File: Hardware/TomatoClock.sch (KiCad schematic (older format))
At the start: 26 parts, among them J1 Boot, J2 UART, J3 USB_B_Micro, J4 Ultrasonic, J5 Buttons, J6 Battery, Q1 S9014, U1 STM32F103C8T6, U2 WS4518E, U3 AP1117-33, Y1 8MHz, Y2 32.768kHz

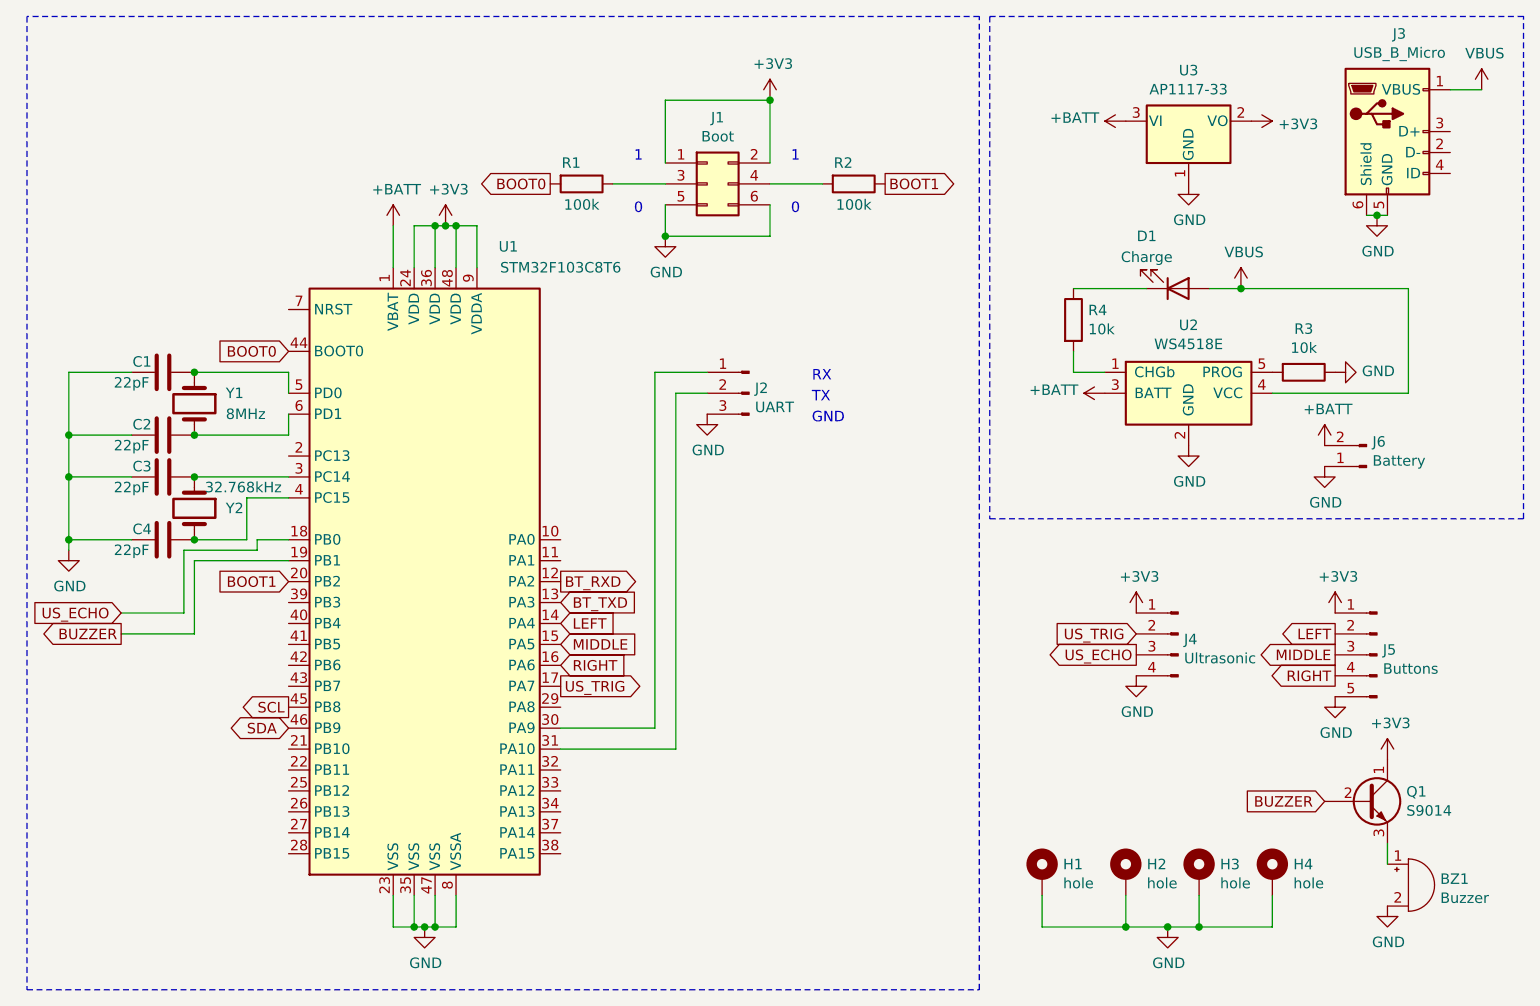
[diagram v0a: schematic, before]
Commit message: Hardware: Update PCB and schematics
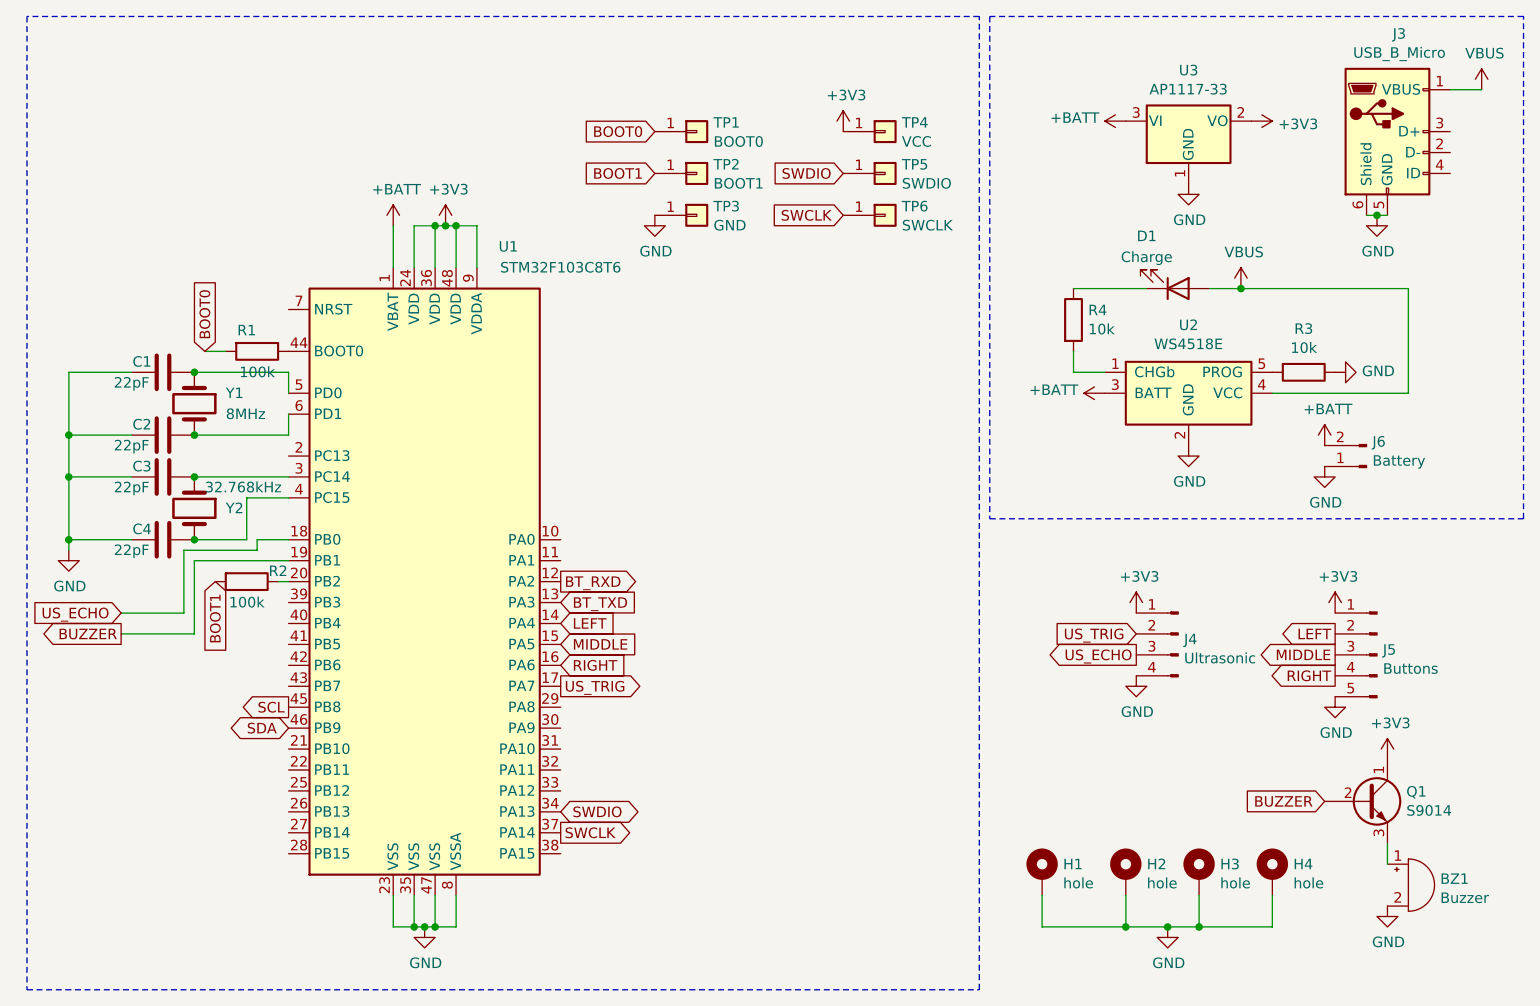
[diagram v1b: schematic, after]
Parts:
- removed J1: Boot, Connector_PinHeader_2.00mm:PinHeader_2x03_P2.00mm_Vertical, symbol Connector_Generic:Conn_02x03_Odd_Even
- removed J2: UART, Connector_PinHeader_2.00mm:PinHeader_1x03_P2.00mm_Vertical, symbol Connector:Conn_01x03_Male
- added TP1: BOOT0, TestPoint:TestPoint_Pad_D1.5mm, symbol Connector_Generic:Conn_01x01
- added TP2: BOOT1, TestPoint:TestPoint_Pad_D1.5mm, symbol Connector_Generic:Conn_01x01
- added TP3: GND, TestPoint:TestPoint_Pad_D1.5mm, symbol Connector_Generic:Conn_01x01
- added TP4: VCC, TestPoint:TestPoint_Pad_D1.5mm, symbol Connector_Generic:Conn_01x01
- added TP5: SWDIO, TestPoint:TestPoint_Pad_D1.5mm, symbol Connector_Generic:Conn_01x01
- added TP6: SWCLK, TestPoint:TestPoint_Pad_D1.5mm, symbol Connector_Generic:Conn_01x01
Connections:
- net +3V3: now also TP4.1 (Pin_1)
- net BOOT0: now also TP1.1 (Pin_1); no longer U1.44 (BOOT0)
- net BOOT1: now also R2.2, TP2.1 (Pin_1); no longer R2.1, U1.20 (PB2)
- net GND: now also TP3.1 (Pin_1)
- net SWDIO: now reaches U1.34 (PA13)
- net SWDIO: now also TP5.1 (Pin_1)
- net SWCLK: now reaches U1.37 (PA14)
- net SWCLK: now also TP6.1 (Pin_1)
- net at R1.1: now also U1.44 (BOOT0)
- new net: R2.1, U1.20 (PB2)
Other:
- note removed: "0"
- note removed: "1"
- note removed: "GND"
- note removed: "RX"
- note removed: "TX"
- moved on the sheet: R1
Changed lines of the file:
@@
 	1600 3050 1350 3050
 Connection ~ 1350 3050
-Text GLabel 1800 2150 0    50   Input ~ 0
+Text GLabel 1400 2150 1    50   Input ~ 0
 BOOT0
-Text GLabel 1800 3250 0    50   Input ~ 0
+Text GLabel 1450 3250 3    50   Input ~ 0
 BOOT1
-$Comp
-L Device:R R2
-U 1 1 61A5B290
-P 4500 1350
-F 0 "R2" V 4400 1300 50  0000 C CNN
-F 1 "100k" V 4600 1350 50  0000 C CNN
-F 2 "Resistor_SMD:R_0603_1608Metric" V 4430 1350 50  0001 C CNN
-F 3 "~" H 4500 1350 50  0001 C CNN
-	1    4500 1350
-	0    1    1    0
-$EndComp
-Wire Wire Line
-	3350 1350 3600 1350
-Wire Wire Line
-	4100 1350 4350 1350
-Text GLabel 3050 1350 0    50   Output ~ 0
-BOOT0
-Text GLabel 4650 1350 2    50   Output ~ 0
-BOOT1
-$Comp
-L power:+3V3 #PWR06
-U 1 1 61A612C6
-P 4100 950
-F 0 "#PWR06" H 4100 800 50  0001 C CNN
-F 1 "+3V3" H 4115 1123 50  0000 C CNN
-F 2 "" H 4100 950 50  0001 C CNN
-F 3 "" H 4100 950 50  0001 C CNN
-	1    4100 950
-	1    0    0    -1
-$EndComp
-Wire Wire Line
-	4100 950  4100 1250
-Wire Wire Line
-	4100 950  3600 950
-Wire Wire Line
-	3600 950  3600 1250
-Connection ~ 4100 950
-$Comp
-L power:GND #PWR05
-U 1 1 61A66348
-P 3600 1600
-F 0 "#PWR05" H 3600 1350 50  0001 C CNN
-F 1 "GND" H 3605 1427 50  0000 C CNN
-F 2 "" H 3600 1600 50  0001 C CNN
-F 3 "" H 3600 1600 50  0001 C CNN
-	1    3600 1600
-	1    0    0    -1
-$EndComp
-Wire Wire Line
-	3600 1450 3600 1600
-Wire Wire Line
-	4100 1450 4100 1600
-Wire Wire Line
-	4100 1600 3600 1600
-Connection ~ 3600 1600
 $Comp
 L Regulator_Linear:AP1117-33 U3
@@
 	1    0    0    -1
 $EndComp
-$Comp
-L Connector:Conn_01x03_Male J2
-U 1 1 61A91DE9
-P 4000 2350
-F 0 "J2" H 3972 2374 50  0000 R CNN
-F 1 "UART" H 3972 2283 50  0000 R CNN
-F 2 "Connector_PinHeader_2.00mm:PinHeader_1x03_P2.00mm_Vertical" H 4000 2350 50  0001 C CNN
-F 3 "~" H 4000 2350 50  0001 C CNN
-	1    4000 2350
-	-1   0    0    -1
-$EndComp
-$Comp
-L power:GND #PWR014
-U 1 1 61A954C1
-P 3800 2450
-F 0 "#PWR014" H 3800 2200 50  0001 C CNN
-F 1 "GND" H 3805 2277 50  0000 C CNN
-F 2 "" H 3800 2450 50  0001 C CNN
-F 3 "" H 3800 2450 50  0001 C CNN
-	1    3800 2450
-	1    0    0    -1
-$EndComp
-Text Notes 3450 1500 0    50   ~ 0
-0
-Text Notes 3450 1250 0    50   ~ 0
-1
-Text Notes 4200 1500 0    50   ~ 0
-0
-Text Notes 4200 1250 0    50   ~ 0
-1
-Wire Wire Line
-	3100 3950 3550 3950
-Wire Wire Line
-	3550 3950 3550 2250
-Wire Wire Line
-	3550 2250 3800 2250
-Wire Wire Line
-	3800 2350 3650 2350
-Wire Wire Line
-	3650 2350 3650 4050
-Wire Wire Line
-	3650 4050 3100 4050
-Text Notes 4300 2300 0    50   ~ 0
-RX
-Text Notes 4300 2400 0    50   ~ 0
-TX
-Text Notes 4300 2500 0    50   ~ 0
-GND
 Wire Notes Line
 	550  550  550  5200
@@
 L Device:R R1
 U 1 1 61A5A591
-P 3200 1350
-F 0 "R1" V 3100 1300 50  0000 C CNN
-F 1 "100k" V 3300 1350 50  0000 C CNN
-F 2 "Resistor_SMD:R_0603_1608Metric" V 3130 1350 50  0001 C CNN
-F 3 "~" H 3200 1350 50  0001 C CNN
-	1    3200 1350
+P 1650 2150
+F 0 "R1" V 1550 2100 50  0000 C CNN
+F 1 "100k" V 1750 2150 50  0000 C CNN
+F 2 "Resistor_SMD:R_0603_1608Metric" V 1580 2150 50  0001 C CNN
+F 3 "~" H 1650 2150 50  0001 C CNN
+	1    1650 2150
 	0    1    1    0
-$EndComp
-$Comp
-L Connector_Generic:Conn_02x03_Odd_Even J1
-U 1 1 61ACA0B6
-P 3800 1350
-F 0 "J1" H 3850 1667 50  0000 C CNN
-F 1 "Boot" H 3850 1576 50  0000 C CNN
-F 2 "Connector_PinHeader_2.00mm:PinHeader_2x03_P2.00mm_Vertical" H 3800 1350 50  0001 C CNN
-F 3 "~" H 3800 1350 50  0001 C CNN
-	1    3800 1350
-	1    0    0    -1
 $EndComp
 $Comp
@@
 	1    0    0    -1
 $EndComp
+Wire Wire Line
+	1500 2150 1400 2150
+$Comp
+L Device:R R2
+U 1 1 61C1663A
+P 1600 3250
+F 0 "R2" V 1550 3400 50  0000 C CNN
+F 1 "100k" V 1700 3250 50  0000 C CNN
+F 2 "Resistor_SMD:R_0603_1608Metric" V 1530 3250 50  0001 C CNN
+F 3 "~" H 1600 3250 50  0001 C CNN
+	1    1600 3250
+	0    1    1    0
+$EndComp
+Wire Wire Line
+	1800 3250 1750 3250
+$Comp
+L Connector_Generic:Conn_01x01 TP1
+U 1 1 61BF10E0
+P 3750 1100
+F 0 "TP1" H 3830 1142 50  0000 L CNN
+F 1 "BOOT0" H 3830 1051 50  0000 L CNN
+F 2 "TestPoint:TestPoint_Pad_D1.5mm" H 3750 1100 50  0001 C CNN
+F 3 "~" H 3750 1100 50  0001 C CNN
+	1    3750 1100
+	1    0    0    -1
+$EndComp
+Text GLabel 3550 1100 0    50   Input ~ 0
+BOOT0
+$Comp
+L Connector_Generic:Conn_01x01 TP2
+U 1 1 61BF32BB
+P 3750 1300
+F 0 "TP2" H 3830 1342 50  0000 L CNN
+F 1 "BOOT1" H 3830 1251 50  0000 L CNN
+F 2 "TestPoint:TestPoint_Pad_D1.5mm" H 3750 1300 50  0001 C CNN
+F 3 "~" H 3750 1300 50  0001 C CNN
+	1    3750 1300
+	1    0    0    -1
+$EndComp
+Text GLabel 3550 1300 0    50   Input ~ 0
+BOOT1
+$Comp
+L Connector_Generic:Conn_01x01 TP3
+U 1 1 61BF5138
+P 3750 1500
+F 0 "TP3" H 3830 1542 50  0000 L CNN
+F 1 "GND" H 3830 1451 50  0000 L CNN
+F 2 "TestPoint:TestPoint_Pad_D1.5mm" H 3750 1500 50  0001 C CNN
+F 3 "~" H 3750 1500 50  0001 C CNN
+	1    3750 1500
+	1    0    0    -1
+$EndComp
+$Comp
+L power:GND #PWR05
+U 1 1 61BF6FB1
+P 3550 1500
+F 0 "#PWR05" H 3550 1250 50  0001 C CNN
+F 1 "GND" H 3555 1327 50  0000 C CNN
+F 2 "" H 3550 1500 50  0001 C CNN
+F 3 "" H 3550 1500 50  0001 C CNN
+	1    3550 1500
+	1    0    0    -1
+$EndComp
+$Comp
+L Connector_Generic:Conn_01x01 TP4
+U 1 1 61BF77FB
+P 4650 1100
+F 0 "TP4" H 4730 1142 50  0000 L CNN
+F 1 "VCC" H 4730 1051 50  0000 L CNN
+F 2 "TestPoint:TestPoint_Pad_D1.5mm" H 4650 1100 50  0001 C CNN
+F 3 "~" H 4650 1100 50  0001 C CNN
+	1    4650 1100
+	1    0    0    -1
+$EndComp
+$Comp
+L power:+3V3 #PWR06
+U 1 1 61BF9632
+P 4450 1100
+F 0 "#PWR06" H 4450 950 50  0001 C CNN
+F 1 "+3V3" H 4465 1273 50  0000 C CNN
+F 2 "" H 4450 1100 50  0001 C CNN
+F 3 "" H 4450 1100 50  0001 C CNN
+	1    4450 1100
+	1    0    0    -1
+$EndComp
+Text GLabel 3100 4350 2    50   BiDi ~ 0
+SWDIO
+Text GLabel 3100 4450 2    50   Output ~ 0
+SWCLK
+$Comp
+L Connector_Generic:Conn_01x01 TP5
+U 1 1 61BF3A3F
+P 4650 1300
+F 0 "TP5" H 4730 1342 50  0000 L CNN
+F 1 "SWDIO" H 4730 1251 50  0000 L CNN
+F 2 "TestPoint:TestPoint_Pad_D1.5mm" H 4650 1300 50  0001 C CNN
+F 3 "~" H 4650 1300 50  0001 C CNN
+	1    4650 1300
+	1    0    0    -1
+$EndComp
+Text GLabel 4450 1300 0    50   Input ~ 0
+SWDIO
+$Comp
+L Connector_Generic:Conn_01x01 TP6
+U 1 1 61BF57EE
+P 4650 1500
+F 0 "TP6" H 4730 1542 50  0000 L CNN
+F 1 "SWCLK" H 4730 1451 50  0000 L CNN
+F 2 "TestPoint:TestPoint_Pad_D1.5mm" H 4650 1500 50  0001 C CNN
+F 3 "~" H 4650 1500 50  0001 C CNN
+	1    4650 1500
+	1    0    0    -1
+$EndComp
+Text GLabel 4450 1500 0    50   Input ~ 0
+SWCLK
 $EndSCHEMATC

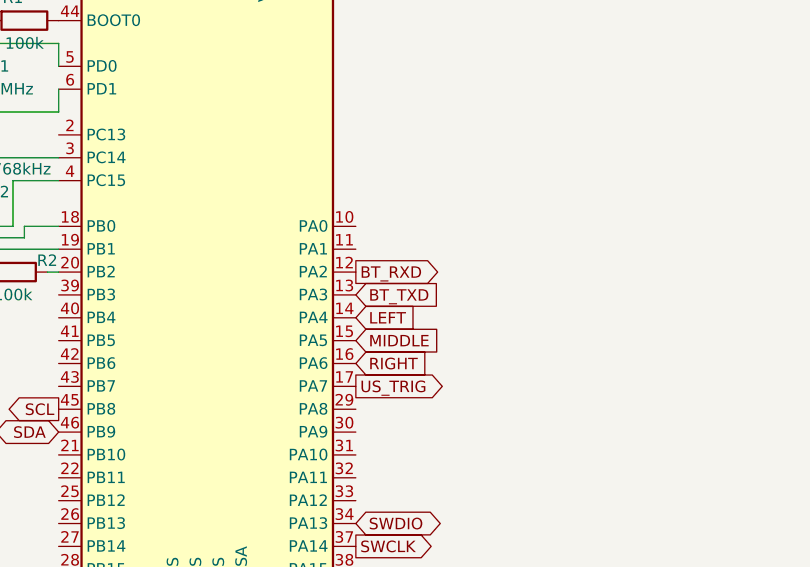
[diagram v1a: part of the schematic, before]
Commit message: Hardware: Update hardware
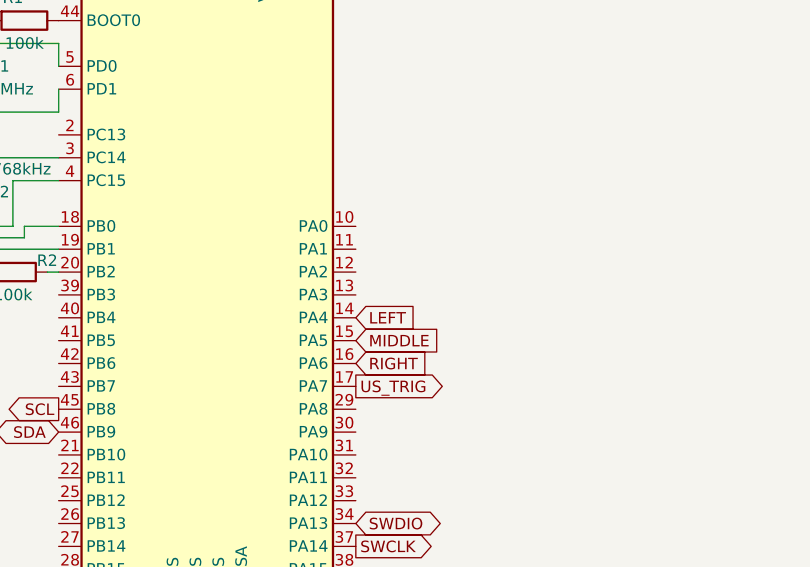
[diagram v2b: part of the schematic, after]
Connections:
- net BT_RXD: no longer names the net of U1.12 (PA2)
- net BT_TXD: no longer names the net of U1.13 (PA3)
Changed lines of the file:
@@
 Text GLabel 6800 3700 0    50   Output ~ 0
 RIGHT
-Text GLabel 3100 3250 2    50   Output ~ 0
-BT_RXD
-Text GLabel 3100 3350 2    50   Input ~ 0
-BT_TXD
 Text GLabel 3100 3450 2    50   Input ~ 0
 LEFT
